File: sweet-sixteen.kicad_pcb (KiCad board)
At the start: 2 copper layers, 115 x 105 mm, 83 parts, among them P1 SDA_I, P10 VIN_O, P11 GND_O, P12 SDA_O, P13 CLK_O, P14 LE_O, P15 ~OE_O, P2 CLK_I, P3 LE_I, P4 ~OE_I, P5 CONN_02X20, P6 5V_I, P7 VIN_I, P8 GND_I, P9 5V_O, U1 STP16CPC26, U2 STP16CPC26, U20 OKI-T/3-W40, U21 OKI-T/3-W40, U3 STP16CPC26, U30 74HCT08, U31 74HCT08, U4 STP16CPC26, U5 STP16CPC26, U6 STP16CPC26, U7 STP16CPC26, U8 STP16CPC26, U9 STP16CPC26

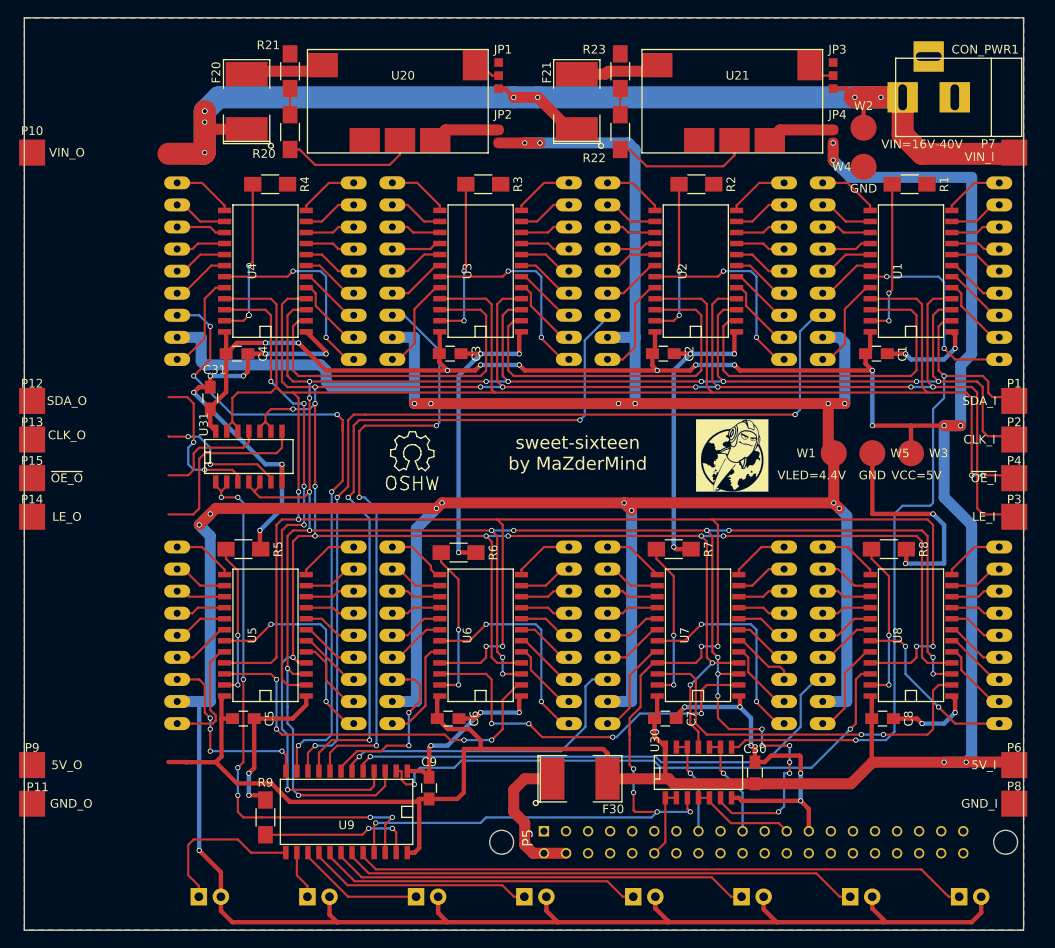
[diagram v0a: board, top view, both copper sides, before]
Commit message: reposition everything, rip up everything… meeeh…
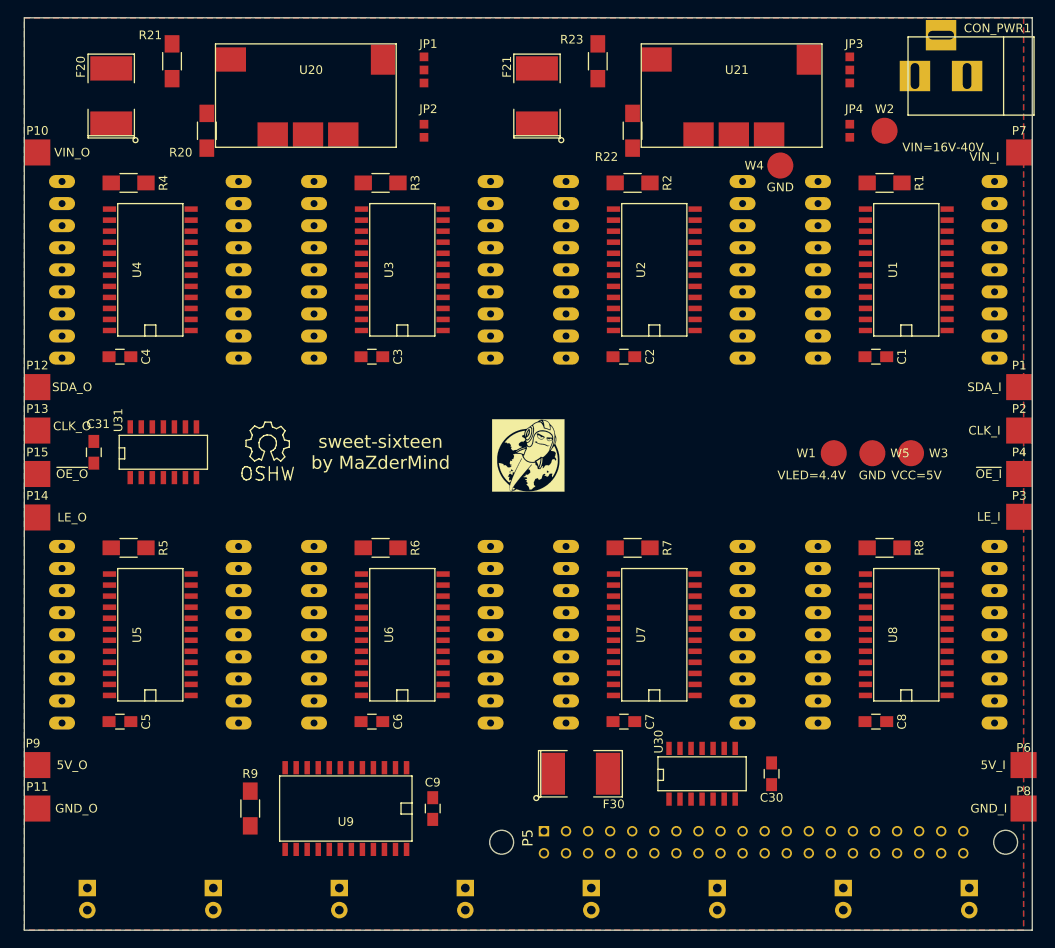
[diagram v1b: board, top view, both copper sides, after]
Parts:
- moved G*** 23.5 mm to (158.0, 100.4)
- moved ? 16.7 mm to (128.0, 99.0)
- moved R4 16.3 mm to (112.0, 69.0)
- moved F20 15.6 mm to (110.0, 59.0)
- moved C31 14.8 mm to (108.0, 100.0)
- moved C5 14.2 mm to (111.0, 131.0)
- moved R21 13.6 mm to (117.0, 55.0)
- moved C4 13.5 mm to (111.0, 89.0)
- moved AFF4 13.2 mm to (114.5, 79.0)
- moved U4 13.2 mm to (114.5, 79.0)
- moved AFF5 13.2 mm to (114.5, 121.0)
- moved U5 13.2 mm to (114.5, 121.0)
- moved R5 13.2 mm to (112.0, 111.0)
- moved D1 12.9 mm to (107.2, 150.1), turned to 270 degrees
- moved R3 11.8 mm to (141.0, 69.0)
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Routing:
- net /VLED: track 485.2 -> 0.00 mm, vias 17 -> 0
- net /~OE: track 416.7 -> 0.00 mm, vias 15 -> 0
- net VCC: track 370.2 -> 0.00 mm, vias 16 -> 0
- net /CLK: track 363.9 -> 0.00 mm, vias 29 -> 0
- net /LE: track 356.7 -> 0.00 mm, vias 19 -> 0
- net GND: track 247.0 -> 0.00 mm, vias 29 -> 0
- net VIN: track 140.5 -> 0.00 mm, vias 8 -> 0
- net Net-(AFF1-Pad12): track 108.3 -> 0.00 mm, vias 3 -> 0
- net Net-(AFF2-Pad12): track 85.7 -> 0.00 mm, vias 3 -> 0
- net /SDA_I: track 81.5 -> 0.00 mm, vias 2 -> 0
- net Net-(AFF4-Pad12): track 74.8 -> 0.00 mm, vias 5 -> 0
- net Net-(D8-Pad1): track 71.0 -> 0.00 mm
- net Net-(AFF3-Pad12): track 70.6 -> 0.00 mm, vias 3 -> 0
- net /SDA_89: track 65.4 -> 0.00 mm, vias 2 -> 0
- net /SDA_O: track 64.5 -> 0.00 mm, vias 7 -> 0
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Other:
- board size 115 x 105 mm -> 116 x 105 mm
